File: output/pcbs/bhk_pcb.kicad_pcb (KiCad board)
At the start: 2 copper layers, 168.2 x 127.4 mm, 115 parts

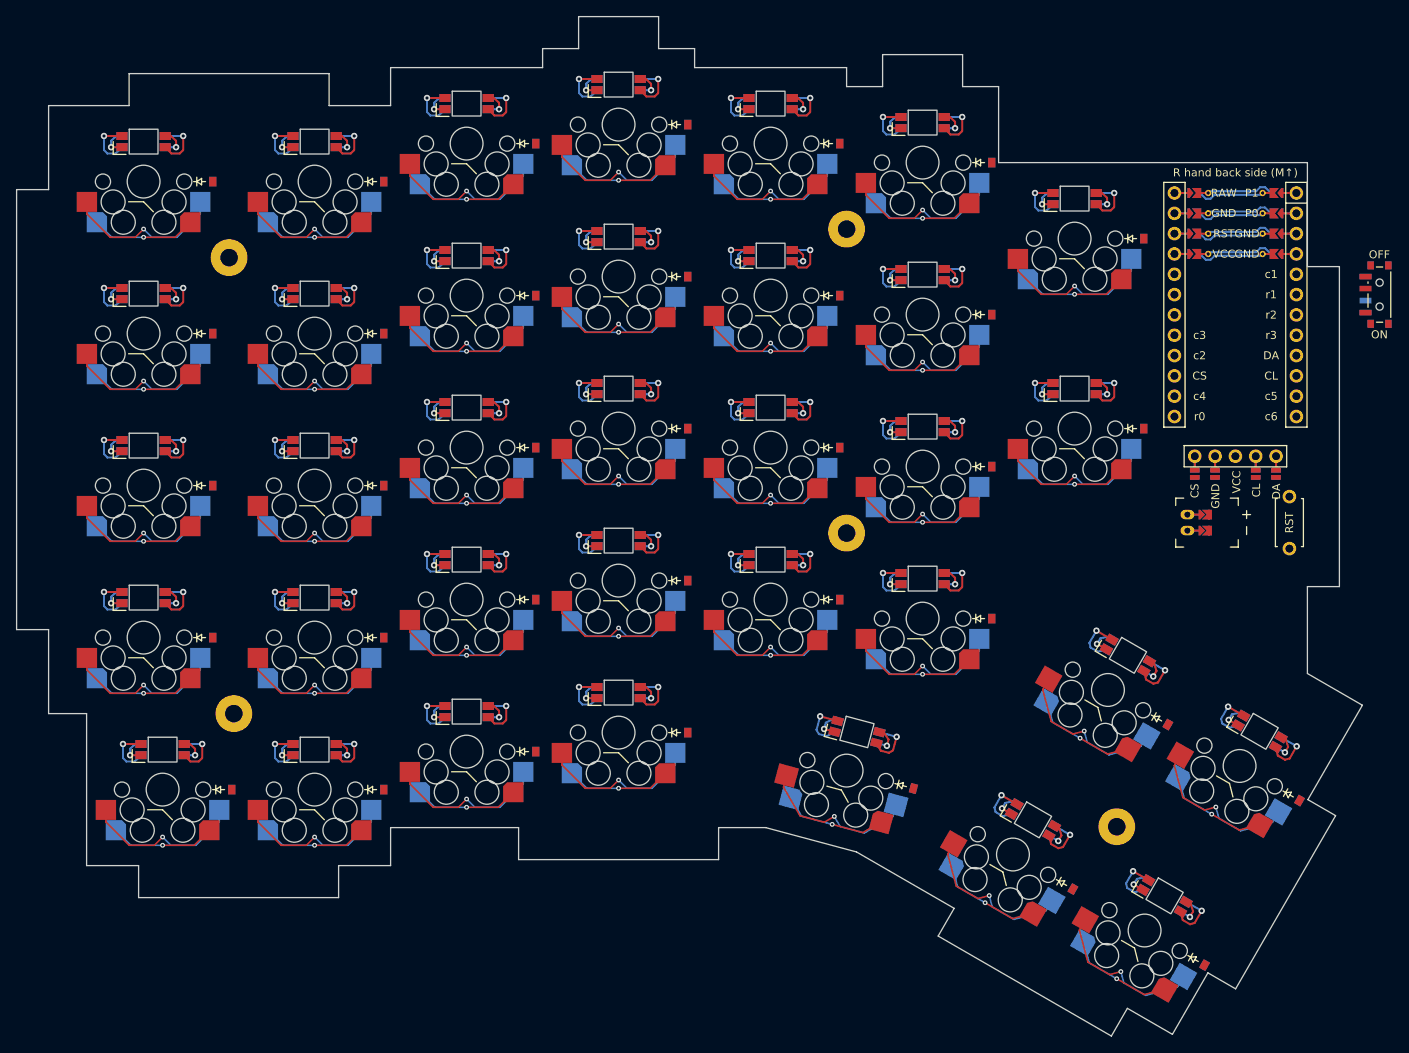
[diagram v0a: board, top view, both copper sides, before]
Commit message: update to pcb layout
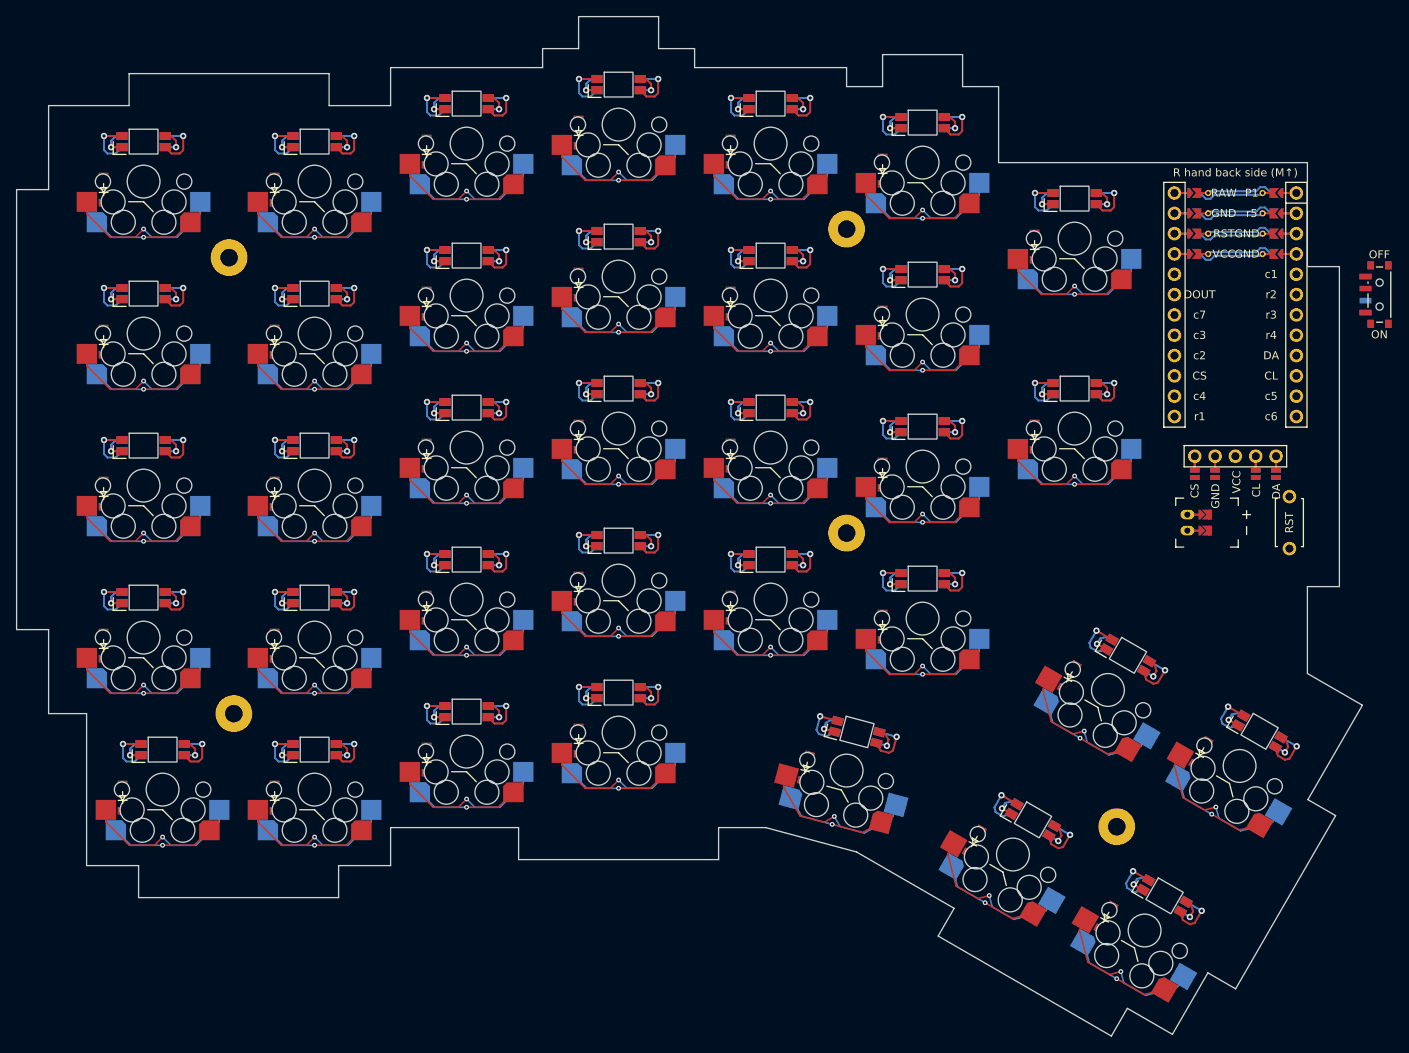
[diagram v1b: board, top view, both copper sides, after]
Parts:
- moved D31 12.0 mm to (232.8, 147.3), turned to 75 degrees
- moved D1 12.0 mm to (147.4, 151.0), turned to 90 degrees
- moved D10 12.0 mm to (166.4, 75.0), turned to 90 degrees
- moved D11 12.0 mm to (185.4, 146.2), turned to 90 degrees
- moved D12 12.0 mm to (185.4, 127.2), turned to 90 degrees
- moved D13 12.0 mm to (185.4, 108.2), turned to 90 degrees
- moved D14 12.0 mm to (185.4, 89.2), turned to 90 degrees
- moved D15 12.0 mm to (185.4, 70.2), turned to 90 degrees
- moved D16 12.0 mm to (204.4, 143.9), turned to 90 degrees
- moved D17 12.0 mm to (204.4, 124.9), turned to 90 degrees
- moved D18 12.0 mm to (204.4, 105.9), turned to 90 degrees
- moved D19 12.0 mm to (204.4, 86.9), turned to 90 degrees
- moved D2 12.0 mm to (145.0, 132.0), turned to 90 degrees
- moved D20 12.0 mm to (204.4, 67.9), turned to 90 degrees
- moved D21 12.0 mm to (223.4, 127.2), turned to 90 degrees
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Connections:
- D31 pad 1: r2 -> r5
- D32 pad 1: r2 -> r5
- D33 pad 1: r1 -> r3
- D34 pad 1: r2 -> r5
- D35 pad 1: r1 -> r4
- LED1 pad 2: LED_END -> LED_27
- LED1 pad 4: LED_34 -> LED_26
- LED10 pad 2: LED_27 -> LED_6
- LED10 pad 4: LED_25 -> LED_5
- LED11 pad 2: LED_26 -> LED_29
- LED11 pad 4: LED_24 -> LED_28
- LED12 pad 2: LED_25 -> LED_23
- LED12 pad 4: LED_23 -> LED_22
- LED13 pad 2: LED_24 -> LED_17
- LED13 pad 4: LED_22 -> LED_16
- LED14 pad 2: LED_23 -> LED_10
- LED14 pad 4: LED_21 -> LED_9
- LED15 pad 2: LED_22 -> LED_5
- LED15 pad 4: LED_20 -> LED_4
- LED16 pad 2: LED_21 -> LED_30
- LED16 pad 4: LED_19 -> LED_29
- LED17 pad 2: LED_20 -> LED_24
- LED17 pad 4: LED_18 -> LED_23
- LED18 pad 2: LED_19 -> LED_18
- LED19 pad 2: LED_18 -> LED_11
- LED19 pad 4: LED_16 -> LED_10
- LED2 pad 2: LED_35 -> LED_21
- LED2 pad 4: LED_33 -> LED_20
- LED20 pad 2: LED_17 -> LED_4
- LED20 pad 4: LED_15 -> LED_3
- LED21 pad 2: LED_16 -> LED_25
- LED21 pad 4: LED_14 -> LED_24
- LED22 pad 2: LED_15 -> LED_19
- LED22 pad 4: LED_13 -> LED_18
- LED23 pad 2: LED_14 -> LED_12
- LED23 pad 4: LED_12 -> LED_11
- LED24 pad 2: LED_13 -> LED_3
- LED24 pad 4: LED_11 -> LED_2
- LED25 pad 2: LED_11 -> LED_26
- LED25 pad 4: LED_9 -> LED_25
- LED26 pad 2: LED_10 -> LED_20
- LED26 pad 4: LED_8 -> LED_19
- LED27 pad 2: LED_9 -> LED_13
- LED27 pad 4: LED_7 -> LED_12
- LED28 pad 2: LED_8 -> LED_2
- LED28 pad 4: LED_6 -> LED_1
- LED29 pad 2: LED_3 -> LED_14
- LED29 pad 4: LED_1 -> LED_13
- LED3 pad 2: LED_34 -> LED_15
- LED3 pad 4: LED_32 -> LED_14
- LED30 pad 2: LED_2 -> LED_1
- LED30 pad 4: LED -> DOUT
- LED31 pad 2: LED_12 -> LED_31
- LED31 pad 4: LED_10 -> LED_30
- LED32 pad 2: LED_6 -> LED_32
- LED32 pad 4: LED_4 -> LED_31
- LED33 pad 2: LED_7 -> LED_33
- LED33 pad 4: LED_5 -> LED_32
- LED34 pad 2: LED_4 -> LED_34
- LED34 pad 4: LED_2 -> LED_33
- LED35 pad 2: LED_5 -> LED_END
- LED35 pad 4: LED_3 -> LED_34
- LED4 pad 2: LED_33 -> LED_8
- LED4 pad 4: LED_31 -> LED_7
- LED5 pad 2: LED_32 -> LED_7
- LED5 pad 4: LED_30 -> LED_6
- LED6 pad 2: LED_31 -> LED_28
- LED6 pad 4: LED_29 -> LED_27
- LED7 pad 2: LED_30 -> LED_22
- LED7 pad 4: LED_28 -> LED_21
- LED8 pad 2: LED_29 -> LED_16
- LED8 pad 4: LED_27 -> LED_15
- LED9 pad 2: LED_28 -> LED_9
- LED9 pad 4: LED_26 -> LED_8
- MCU1 pad 102: P0 -> r5
- MCU1 pad 13: r0 -> r1
- MCU1 pad 18: P19 -> c7
- MCU1 pad 19: P20 -> DOUT
- MCU1 pad 6: r1 -> r2
- MCU1 pad 7: r2 -> r3
- MCU1 pad 8: r3 -> r4
- S1 pad 1: c1_r5 -> c1
- S1 pad 2: c1 -> c1_r5
- S10 pad 1: c2_r1 -> c2
- S10 pad 2: c2 -> c2_r1
- S11 pad 1: c3_r5 -> c3
- S11 pad 2: c3 -> c3_r5
- S12 pad 1: c3_r4 -> c3
- S12 pad 2: c3 -> c3_r4
- S13 pad 1: c3_r3 -> c3
- S13 pad 2: c3 -> c3_r3
- S14 pad 1: c3_r2 -> c3
- S14 pad 2: c3 -> c3_r2
- S15 pad 1: c3_r1 -> c3
- S15 pad 2: c3 -> c3_r1
- S16 pad 1: c4_r5 -> c4
- S16 pad 2: c4 -> c4_r5
- S17 pad 1: c4_r4 -> c4
- S17 pad 2: c4 -> c4_r4
- S18 pad 1: c4_r3 -> c4
- S18 pad 2: c4 -> c4_r3
- S19 pad 1: c4_r2 -> c4
- S19 pad 2: c4 -> c4_r2
- S2 pad 1: c1_r4 -> c1
- S2 pad 2: c1 -> c1_r4
- S20 pad 1: c4_r1 -> c4
- S20 pad 2: c4 -> c4_r1
- S21 pad 1: c5_r4 -> c5
- S21 pad 2: c5 -> c5_r4
- S22 pad 1: c5_r3 -> c5
- S22 pad 2: c5 -> c5_r3
- S23 pad 1: c5_r2 -> c5
- S23 pad 2: c5 -> c5_r2
- S24 pad 1: c5_r1 -> c5
- S24 pad 2: c5 -> c5_r1
- S25 pad 1: c6_r4 -> c6
- S25 pad 2: c6 -> c6_r4
- S26 pad 1: c6_r3 -> c6
- S26 pad 2: c6 -> c6_r3
- S27 pad 1: c6_r2 -> c6
- S27 pad 2: c6 -> c6_r2
- S28 pad 1: c6_r1 -> c6
- S28 pad 2: c6 -> c6_r1
- S29 pad 1: c7_r2 -> c7
- S29 pad 2: c7 -> c7_r2
- S3 pad 1: c1_r3 -> c1
- S3 pad 2: c1 -> c1_r3
- S30 pad 1: c7_r1 -> c7
- S30 pad 2: c7 -> c7_r1
- S31 pad 1: c1_r2 -> c5
- S31 pad 2: c1 -> c1_r2
- S32 pad 1: c2_r2 -> c6
- S32 pad 2: c2 -> c2_r2
- S33 pad 1: c2_r1 -> c7
- S33 pad 2: c2 -> c2_r1
- S34 pad 1: c3_r2 -> c7
- S34 pad 2: c3 -> c3_r2
- S35 pad 1: c3_r1 -> c7
- S35 pad 2: c3 -> c3_r1
- S4 pad 1: c1_r2 -> c1
- S4 pad 2: c1 -> c1_r2
- S5 pad 1: c1_r1 -> c1
- S5 pad 2: c1 -> c1_r1
- S6 pad 1: c2_r5 -> c2
- S6 pad 2: c2 -> c2_r5
- S7 pad 1: c2_r4 -> c2
- S7 pad 2: c2 -> c2_r4
- S8 pad 1: c2_r3 -> c2
- S8 pad 2: c2 -> c2_r3
- S9 pad 1: c2_r2 -> c2
- S9 pad 2: c2 -> c2_r2
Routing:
- net c3: track 161.7 -> 52.9 mm, vias 7 -> 5
- net c2: track 161.7 -> 52.9 mm, vias 7 -> 5
- net c1: track 138.6 -> 52.9 mm, vias 6 -> 5
- net c4: track 115.5 -> 52.9 mm
- net c5: track 92.4 -> 52.9 mm, vias 4 -> 5
- net c6: track 92.4 -> 52.9 mm, vias 4 -> 5
- net c3_r2: track 21.2 -> 46.2 mm
- net c3_r1: track 21.2 -> 46.2 mm
- net c2_r1: track 21.2 -> 46.2 mm
- net c2_r2: track 21.2 -> 46.2 mm
- net c1_r2: track 21.2 -> 46.2 mm
- net c6_r4: track 10.6 -> 23.1 mm
- net c5_r4: track 10.6 -> 23.1 mm
- net c4_r5: track 10.6 -> 23.1 mm
- net c3_r5: track 10.6 -> 23.1 mm
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
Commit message: layout and net tweaking
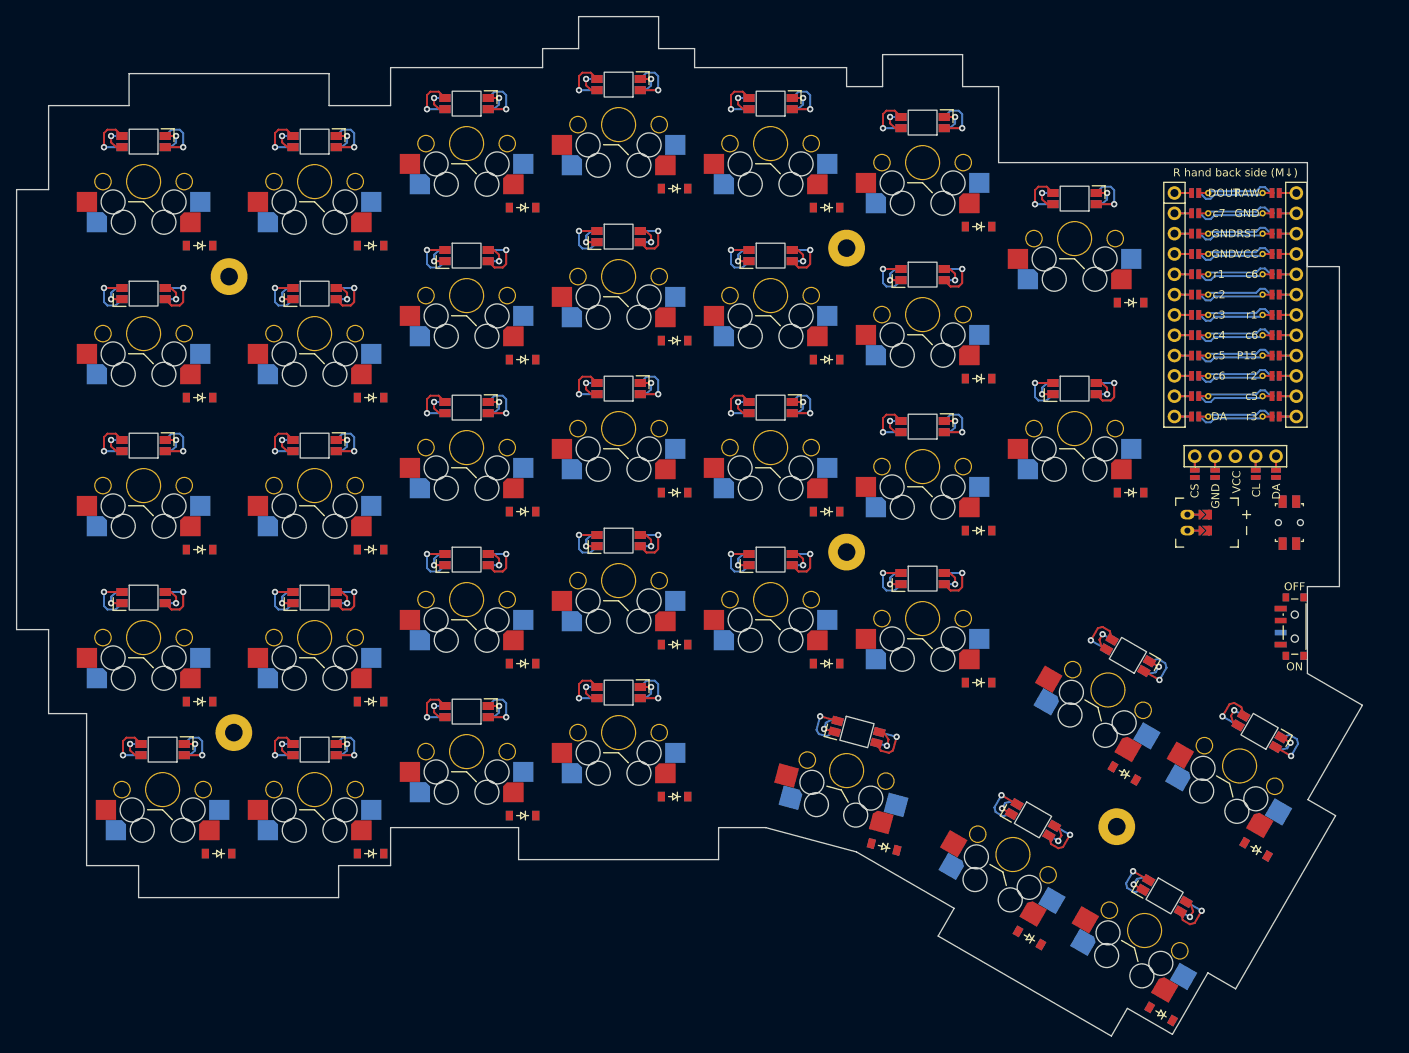
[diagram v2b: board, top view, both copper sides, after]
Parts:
- RST1: footprint ceoloide:reset_switch_tht_top -> ceoloide:reset_switch_smd_side
- moved LED15 114.1 mm to (261.2, 153.8), turned to -30 degrees
- moved LED20 91.4 mm to (171.4, 145.0), turned to 180 degrees
- moved LED32 88.2 mm to (247.4, 66.6), turned to 180 degrees
- moved LED25 82.3 mm to (190.4, 64.2), turned to 180 degrees
- moved LED14 77.0 mm to (239.2, 142.8), turned to -15 degrees
- moved LED13 76.0 mm to (266.4, 99.9)
- moved LED16 72.8 mm to (277.6, 163.3), turned to -30 degrees
- moved LED23 68.5 mm to (190.4, 140.2), turned to 180 degrees
- moved LED12 67.2 mm to (247.4, 85.6)
- moved LED5 66.0 mm to (190.4, 121.2)
- moved LED22 66.0 mm to (171.4, 69.0), turned to 180 degrees
- moved LED9 66.0 mm to (228.4, 121.2)
- moved LED6 64.6 mm to (190.4, 83.2)
- moved LED17 62.7 mm to (152.4, 145.0), turned to 180 degrees
- moved LED19 60.6 mm to (150.0, 69.0), turned to 180 degrees
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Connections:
- net P21 renamed MCU1_20
- LED1 pad 2: LED_27 -> LED_21
- LED1 pad 4: LED_26 -> LED_20
- LED10 pad 2: LED_6 -> LED_12
- LED10 pad 4: LED_5 -> LED_11
- LED11 pad 2: LED_29 -> LED_26
- LED11 pad 4: LED_28 -> LED_25
- LED12 pad 2: LED_23 -> LED_13
- LED12 pad 4: LED_22 -> LED_12
- LED13 pad 2: LED_17 -> LED_14
- LED13 pad 4: LED_16 -> LED_13
- LED14 pad 2: LED_10 -> LED_31
- LED14 pad 4: LED_9 -> LED_30
- LED15 pad 2: LED_5 -> LED_32
- LED15 pad 4: LED_4 -> LED_31
- LED16 pad 2: LED_30 -> LED_34
- LED16 pad 4: LED_29 -> LED_33
- LED17 pad 2: LED_24 -> LED_27
- LED17 pad 4: LED_23 -> LED_26
- LED18 pad 2: LED_18 -> LED_15
- LED18 pad 4: LED_17 -> LED_14
- LED19 pad 2: LED_11 -> LED_7
- LED19 pad 4: LED_10 -> LED_6
- LED2 pad 2: LED_21 -> LED_8
- LED2 pad 4: LED_20 -> LED_7
- LED20 pad 2: LED_4 -> LED_28
- LED20 pad 4: LED_3 -> LED_27
- LED21 pad 2: LED_25 -> LED_16
- LED21 pad 4: LED_24 -> LED_15
- LED22 pad 2: LED_19 -> LED_6
- LED22 pad 4: LED_18 -> LED_5
- LED23 pad 2: LED_12 -> LED_29
- LED23 pad 4: LED_11 -> LED_28
- LED24 pad 2: LED_3 -> LED_17
- LED24 pad 4: LED_2 -> LED_16
- LED25 pad 2: LED_26 -> LED_5
- LED25 pad 4: LED_25 -> LED_4
- LED26 pad 2: LED_20 -> LED_30
- LED26 pad 4: LED_19 -> LED_29
- LED27 pad 2: LED_13 -> LED_18
- LED27 pad 4: LED_12 -> LED_17
- LED28 pad 2: LED_2 -> LED_4
- LED28 pad 4: LED_1 -> LED_3
- LED29 pad 2: LED_14 -> LED_19
- LED29 pad 4: LED_13 -> LED_18
- LED3 pad 2: LED_15 -> LED_22
- LED3 pad 4: LED_14 -> LED_21
- LED30 pad 2: LED_1 -> LED_3
- LED30 pad 4: DOUT -> LED_2
- LED31 pad 2: LED_31 -> LED_20
- LED31 pad 4: LED_30 -> LED_19
- LED32 pad 2: LED_32 -> LED_2
- LED32 pad 4: LED_31 -> LED_1
- LED33 pad 2: LED_33 -> LED_1
- LED33 pad 4: LED_32 -> DOUT
- LED34 pad 2: LED_34 -> LED_33
- LED34 pad 4: LED_33 -> LED_32
- LED4 pad 2: LED_8 -> LED_9
- LED4 pad 4: LED_7 -> LED_8
- LED5 pad 2: LED_7 -> LED_23
- LED5 pad 4: LED_6 -> LED_22
- LED6 pad 2: LED_28 -> LED_10
- LED6 pad 4: LED_27 -> LED_9
- LED7 pad 2: LED_22 -> LED_24
- LED7 pad 4: LED_21 -> LED_23
- LED8 pad 2: LED_16 -> LED_11
- LED8 pad 4: LED_15 -> LED_10
- LED9 pad 2: LED_9 -> LED_25
- LED9 pad 4: LED_8 -> LED_24
- MCU1 pad 10: CL -> MCU1_10
- MCU1 pad 101: P1 -> RAW
- MCU1 pad 102: r5 -> GND
- MCU1 pad 103: GND -> RST
- MCU1 pad 104: GND -> VCC
- MCU1 pad 11: c5 -> MCU1_11
- MCU1 pad 12: c6 -> MCU1_12
- MCU1 pad 121: VCC -> GND
- MCU1 pad 122: RST -> GND
- MCU1 pad 123: GND -> c7
- MCU1 pad 124: RAW -> DOUT
- MCU1 pad 13: r1 -> MCU1_13
- MCU1 pad 14: c4 -> MCU1_14
- MCU1 pad 15: CS -> MCU1_15
- MCU1 pad 16: c2 -> MCU1_16
- MCU1 pad 17: c3 -> MCU1_17
- MCU1 pad 18: c7 -> MCU1_18
- MCU1 pad 19: DOUT -> MCU1_19
- MCU1 pad 5: c1 -> MCU1_5
- MCU1 pad 6: r2 -> MCU1_6
- MCU1 pad 7: r3 -> MCU1_7
- MCU1 pad 8: r4 -> MCU1_8
- MCU1 pad 9: DA -> MCU1_9
- RST1 pad 1: RST -> GND
- RST1 pad 2: GND -> RST
- S1 pad : (no net) -> c1_r5
- S1 pad 1: c1 -> c1_r5
- S1 pad 2: c1_r5 -> c1
- S10 pad : (no net) -> c2_r1
- S10 pad 1: c2 -> c2_r1
- S10 pad 2: c2_r1 -> c2
- S11 pad : (no net) -> c3_r5
- S11 pad 1: c3 -> c3_r5
- S11 pad 2: c3_r5 -> c3
- S12 pad : (no net) -> c3_r4
- S12 pad 1: c3 -> c3_r4
- S12 pad 2: c3_r4 -> c3
- S13 pad : (no net) -> c3_r3
- S13 pad 1: c3 -> c3_r3
- S13 pad 2: c3_r3 -> c3
- S14 pad : (no net) -> c3_r2
- S14 pad 1: c3 -> c3_r2
- S14 pad 2: c3_r2 -> c3
- S15 pad : (no net) -> c3_r1
- S15 pad 1: c3 -> c3_r1
- S15 pad 2: c3_r1 -> c3
- S16 pad : (no net) -> c4_r5
- S16 pad 1: c4 -> c4_r5
- S16 pad 2: c4_r5 -> c4
- S17 pad : (no net) -> c4_r4
- S17 pad 1: c4 -> c4_r4
- S17 pad 2: c4_r4 -> c4
- S18 pad : (no net) -> c4_r3
- S18 pad 1: c4 -> c4_r3
- S18 pad 2: c4_r3 -> c4
- S19 pad : (no net) -> c4_r2
- S19 pad 1: c4 -> c4_r2
- S19 pad 2: c4_r2 -> c4
- S2 pad : (no net) -> c1_r4
- S2 pad 1: c1 -> c1_r4
- S2 pad 2: c1_r4 -> c1
- S20 pad : (no net) -> c4_r1
- S20 pad 1: c4 -> c4_r1
- S20 pad 2: c4_r1 -> c4
- S21 pad : (no net) -> c5_r4
- S21 pad 1: c5 -> c5_r4
- S21 pad 2: c5_r4 -> c5
- S22 pad : (no net) -> c5_r3
- S22 pad 1: c5 -> c5_r3
- S22 pad 2: c5_r3 -> c5
- S23 pad : (no net) -> c5_r2
- S23 pad 1: c5 -> c5_r2
- S23 pad 2: c5_r2 -> c5
- S24 pad : (no net) -> c5_r1
- S24 pad 1: c5 -> c5_r1
- S24 pad 2: c5_r1 -> c5
- S25 pad : (no net) -> c6_r4
- S25 pad 1: c6 -> c6_r4
- S25 pad 2: c6_r4 -> c6
- S26 pad : (no net) -> c6_r3
- S26 pad 1: c6 -> c6_r3
- S26 pad 2: c6_r3 -> c6
- S27 pad : (no net) -> c6_r2
- S27 pad 1: c6 -> c6_r2
- S27 pad 2: c6_r2 -> c6
- S28 pad : (no net) -> c6_r1
- S28 pad 1: c6 -> c6_r1
- S28 pad 2: c6_r1 -> c6
- S29 pad : (no net) -> c7_r2
- S29 pad 1: c7 -> c7_r2
- S29 pad 2: c7_r2 -> c7
- S3 pad : (no net) -> c1_r3
- S3 pad 1: c1 -> c1_r3
- S3 pad 2: c1_r3 -> c1
- S30 pad : (no net) -> c7_r1
- S30 pad 1: c7 -> c7_r1
- S30 pad 2: c7_r1 -> c7
- S31 pad : (no net) -> c1_r2
- S31 pad 1: c5 -> c1_r2
- S31 pad 2: c1_r2 -> c5
- S32 pad : (no net) -> c2_r2
- S32 pad 1: c6 -> c2_r2
- S32 pad 2: c2_r2 -> c6
- S33 pad : (no net) -> c2_r1
- S33 pad 1: c7 -> c2_r1
- S33 pad 2: c2_r1 -> c7
- S34 pad : (no net) -> c3_r2
- S34 pad 1: c7 -> c3_r2
- S34 pad 2: c3_r2 -> c7
- S35 pad : (no net) -> c3_r1
- S35 pad 1: c7 -> c3_r1
- S35 pad 2: c3_r1 -> c7
- S4 pad : (no net) -> c1_r2
- S4 pad 1: c1 -> c1_r2
- S4 pad 2: c1_r2 -> c1
- S5 pad : (no net) -> c1_r1
- S5 pad 1: c1 -> c1_r1
- S5 pad 2: c1_r1 -> c1
- S6 pad : (no net) -> c2_r5
- S6 pad 1: c2 -> c2_r5
- S6 pad 2: c2_r5 -> c2
- S7 pad : (no net) -> c2_r4
- S7 pad 1: c2 -> c2_r4
- S7 pad 2: c2_r4 -> c2
- S8 pad : (no net) -> c2_r3
- S8 pad 1: c2 -> c2_r3
- S8 pad 2: c2_r3 -> c2
- S9 pad : (no net) -> c2_r2
- S9 pad 1: c2 -> c2_r2
- S9 pad 2: c2_r2 -> c2
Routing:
- net (no net): track 112.6 -> 333.1 mm
- net c7: track 52.9 -> 0.00 mm, vias 5 -> 0
- net c6: track 52.9 -> 0.00 mm, vias 5 -> 0
- net c4: track 52.9 -> 0.00 mm, vias 5 -> 0
- net c3: track 52.9 -> 0.00 mm, vias 5 -> 0
- net c2: track 52.9 -> 0.00 mm, vias 5 -> 0
- net c1: track 52.9 -> 0.00 mm, vias 5 -> 0
- net c5: track 52.9 -> 0.00 mm, vias 5 -> 0
- net c3_r2: track 46.2 -> 0.00 mm, vias 2 -> 0
- net c3_r1: track 46.2 -> 0.00 mm, vias 2 -> 0
- net c2_r1: track 46.2 -> 0.00 mm, vias 2 -> 0
- net c2_r2: track 46.2 -> 0.00 mm, vias 2 -> 0
- net c1_r2: track 46.2 -> 0.00 mm, vias 2 -> 0
- net c6_r4: track 23.1 -> 0.00 mm, vias 1 -> 0
- net c5_r4: track 23.1 -> 0.00 mm, vias 1 -> 0
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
